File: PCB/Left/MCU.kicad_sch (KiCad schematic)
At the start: 26 parts, among them J2 , J3 , SW47 SW_Push, U1 XC6220B331MR, U2 BQ24075/9, U3 USBLC6-2SC6, U4 MS88FS3

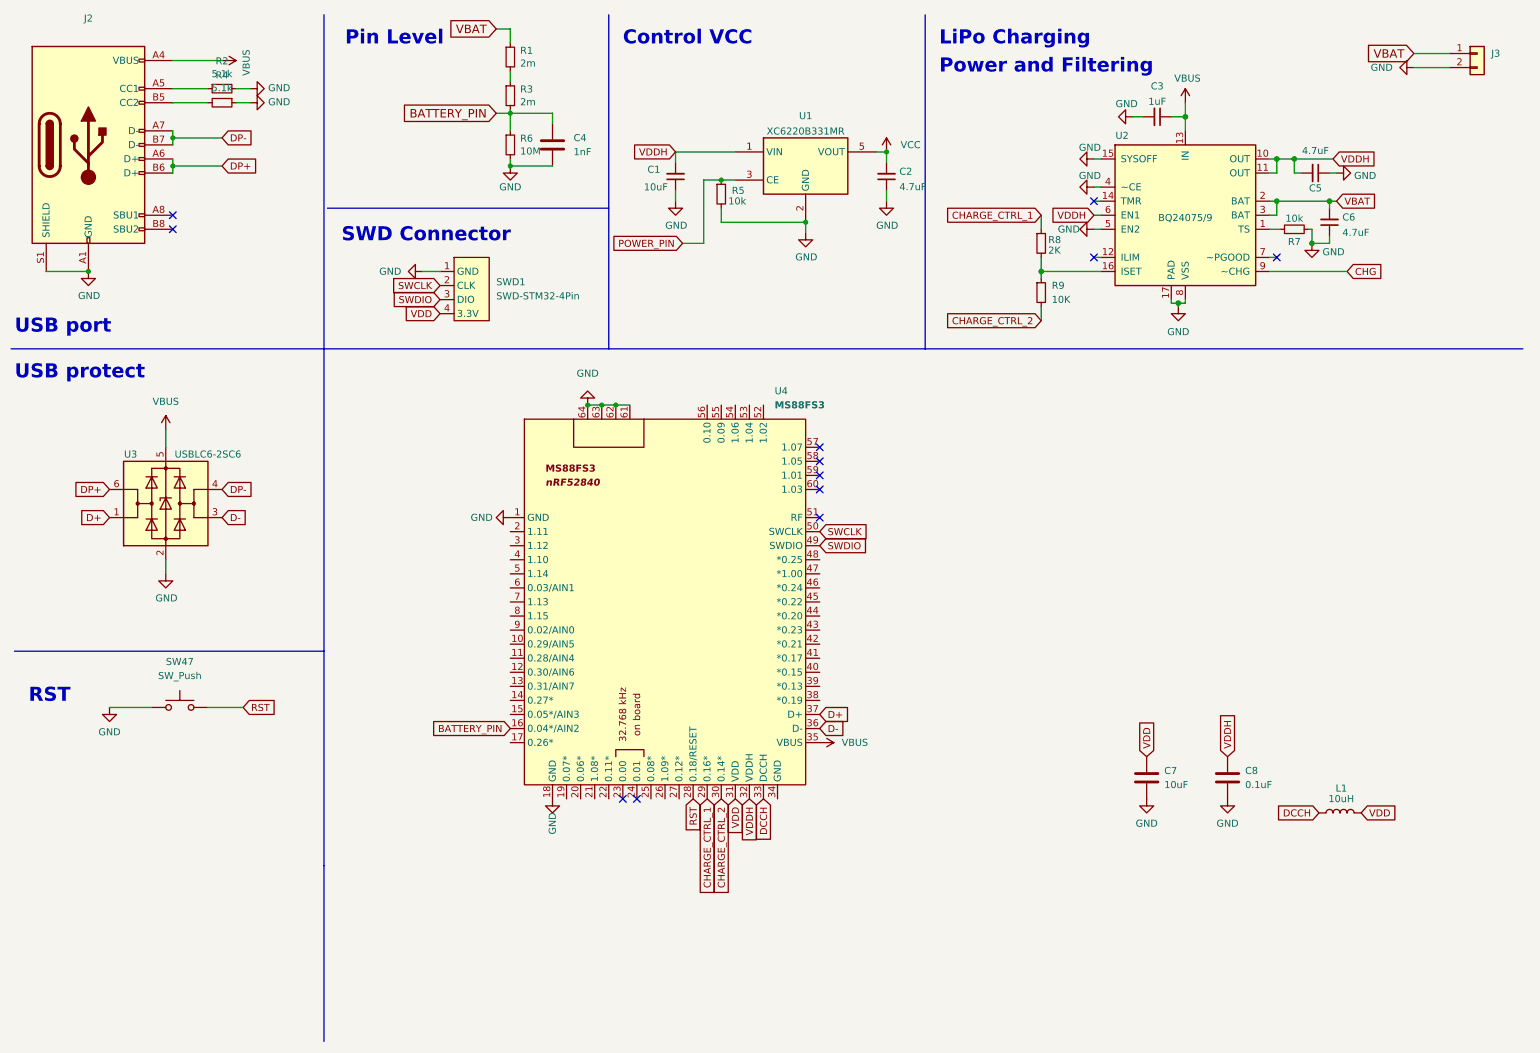
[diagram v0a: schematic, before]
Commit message: cap nhat 16:16 08/06/2022
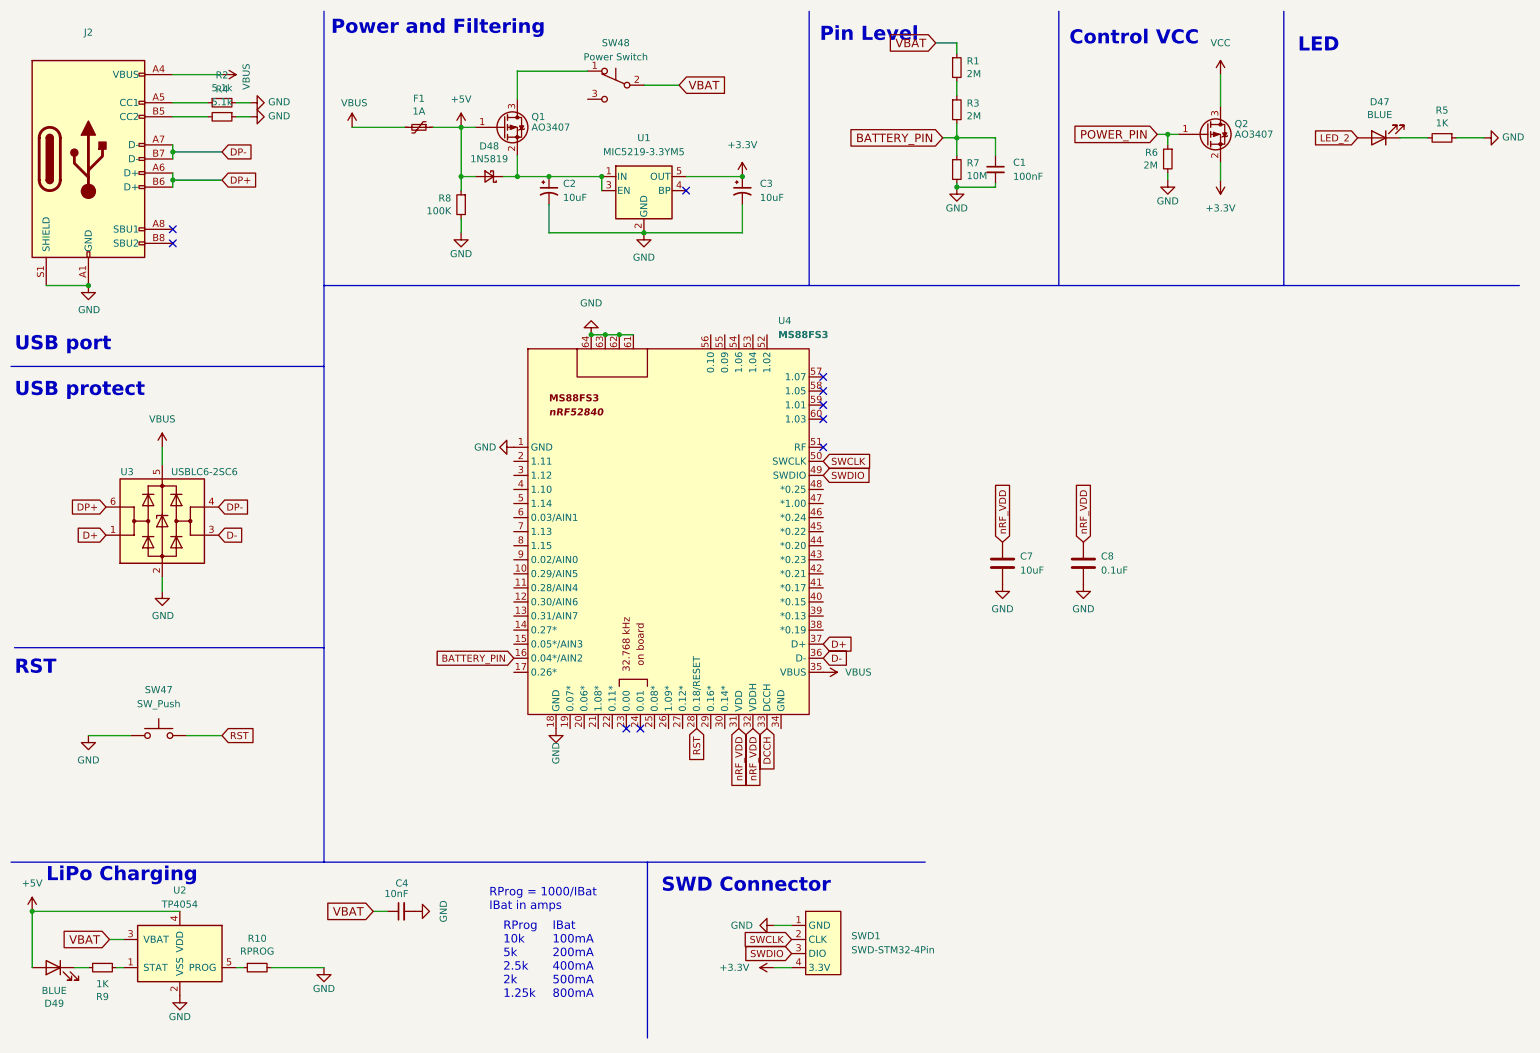
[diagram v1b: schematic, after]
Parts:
- removed C2, C5, C6: 4.7uF, Capacitor_SMD:C_0603_1608Metric_Pad1.08x0.95mm_HandSolder, symbol Device:C_Small
- removed C3: 1uF, Capacitor_SMD:C_0603_1608Metric_Pad1.08x0.95mm_HandSolder, symbol Device:C_Small
- removed C4: 1nF, Capacitor_SMD:C_0603_1608Metric_Pad1.08x0.95mm_HandSolder, symbol Device:C
- removed J3: (no value), kien242:JST_SH_SM02B-SRSS-TB_1x02-1MP, symbol Connector_Generic:Conn_01x02
- removed L1: 10uH, Inductor_SMD:L_0603_1608Metric_Pad1.05x0.95mm_HandSolder, symbol Device:L
- removed U1: XC6220B331MR, Package_TO_SOT_SMD:SOT-23-5, symbol Regulator_Linear:XC6220B331MR
- removed U2: BQ24075/9, kien242:BQ24075, symbol Battery_Management:BQ24075
- added C2, C3: 10uF, Capacitor_Tantalum_SMD:CP_EIA-3216-12_Kemet-S, symbol Device:C_Polarized_Small_US
- added C4: 10nF, Capacitor_SMD:C_0603_1608Metric, symbol Device:C_Small
- added D47, D49: BLUE, LED_SMD:LED_0603_1608Metric_Pad1.05x0.95mm_HandSolder, symbol Device:LED
- added D48: 1N5819, Diode_SMD:D_SOD-323_HandSoldering, symbol Device:D_Schottky_Small
- added F1: 1A, Fuse:Fuse_1206_3216Metric, symbol keeb_parts:Polyfuse_Small
- added Q1, Q2: AO3407, Package_TO_SOT_SMD:SOT-23, symbol Device:Q_PMOS_GSD
- added R10: RPROG, Resistor_SMD:R_0603_1608Metric, symbol Device:R_Small
- added SW48: Power Switch, Button_Switch_SMD:SW_SPDT_PCM12, symbol Switch:SW_Push_SPDT
- added U1: MIC5219-3.3YM5, Package_TO_SOT_SMD:SOT-23-5, symbol Regulator_Linear:MIC5219-3.3YM5
- added U2: TP4054, Package_TO_SOT_SMD:SOT-23-5, symbol Battery_Management:MCP73831-3-OT
- C1: value 10uF -> 100nF; footprint Capacitor_SMD:C_0603_1608Metric_Pad1.08x0.95mm_HandSolder -> Capacitor_SMD:C_0603_1608Metric; JLC Part C19702 -> (none); LCSC Part C19702 -> (none); Manufacturer Part CL10A106KP8NNNC -> (none)
- R1, R3: value 2m -> 2M; footprint Resistor_SMD:R_0603_1608Metric_Pad0.98x0.95mm_HandSolder -> Resistor_SMD:R_0603_1608Metric
- R5: value 10k -> 1K; footprint Resistor_SMD:R_0603_1608Metric_Pad0.98x0.95mm_HandSolder -> Resistor_SMD:R_0603_1608Metric; JLC Part C25744 -> (none); LCSC (none) -> C21190; LCSC Part C60490 -> (none); LCSC Part Number (none) -> C21190; Manufacturer Part RC0402FR-0710KL -> (none)
- R6: value 10M -> 2M; footprint Resistor_SMD:R_0603_1608Metric_Pad0.98x0.95mm_HandSolder -> Resistor_SMD:R_0603_1608Metric
- R7: value 10k -> 10M; footprint Resistor_SMD:R_0603_1608Metric_Pad0.98x0.95mm_HandSolder -> Resistor_SMD:R_0603_1608Metric; JLC Part C25744 -> (none); LCSC Part C60490 -> (none); Manufacturer Part RC0402FR-0710KL -> (none)
- R8: value 2K -> 100K; footprint Resistor_SMD:R_0603_1608Metric_Pad0.98x0.95mm_HandSolder -> Resistor_SMD:R_0603_1608Metric; JLC Part C25744 -> (none); LCSC Part C60490 -> (none); Manufacturer Part RC0402FR-0710KL -> (none)
- R9: value 10K -> 1K; footprint Resistor_SMD:R_0603_1608Metric_Pad0.98x0.95mm_HandSolder -> Resistor_SMD:R_0603_1608Metric; JLC Part C51721 -> (none); LCSC Part C131467 -> (none); Manufacturer Part RC0402FR-073K9L -> (none)
- SWD1: footprint Library:SWD_Connector -> kien242:SWD-4Pin
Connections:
- net BATTERY_PIN: now also C1.1, R7.1; no longer R6.1
- net GND: now also C1.2, R5.1, R8.2, C2.2, C3.2, C4.2, R10.2, U1.2 (GND), U2.2 (VSS); no longer C1.1, R5.2
- net POWER_PIN: now also R6.1, Q2.1 (G); no longer R5.1
- net VBAT: now also C4.1, SW48.2 (B), U2.3 (VBAT)
- net VBUS: now also F1.2
- net VCC: now also Q2.3 (D)
- net at R9.1: now also D49.1 (K); no longer R8.2
- net CHARGE_CTRL_1: no longer names the net of U4.29 (0.16*)
- net CHARGE_CTRL_1: no longer R8.1
- net CHARGE_CTRL_2: no longer names the net of R9.2
- net CHARGE_CTRL_2: now also U2.1 (STAT); no longer U4.30 (0.14*)
- net VDD renamed nRF_VDD
- net nRF_VDD: now also C8.1, U4.32 (VDDH); no longer SWD1.4 (3.3V)
- removed net VDDH: C1.2, C8.1, U4.32 (VDDH)
- new net: C2.1, D48.1 (K), Q1.2 (S), U1.1 (IN), U1.3 (EN)
- new net: Q1.3 (D), SW48.1 (A)
- new net: D47.1 (K), R5.2
- new net: R10.1, U2.5 (PROG)
- new net +3V3: C3.1, Q2.2 (S), SWD1.4 (3.3V), U1.5 (OUT)
- new net +5V: D48.2 (A), D49.2 (A), F1.1, Q1.1 (G), R8.1, U2.4 (VDD)
- new net LED_2: D47.2 (A)
- no-connect marks 12 -> 10
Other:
- note added: "IBat 100mA 200mA 400mA 500mA 800mA"
- note added: "LED"
- note added: "RProg 10k 5k 2.5k 2k 1.25k"
- note added: "RProg = 1000/IBat IBat in amps"
- moved on the sheet: C7, C8, J2, R2, R4, SW47, U3, U4
